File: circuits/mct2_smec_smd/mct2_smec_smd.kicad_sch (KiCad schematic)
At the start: 9 parts, among them J1 Input 1x40 FPC, J2 Conn_01x07, J3 Conn_02x15_Odd_Even, U1 GW1N-UV2QN48C7/I6

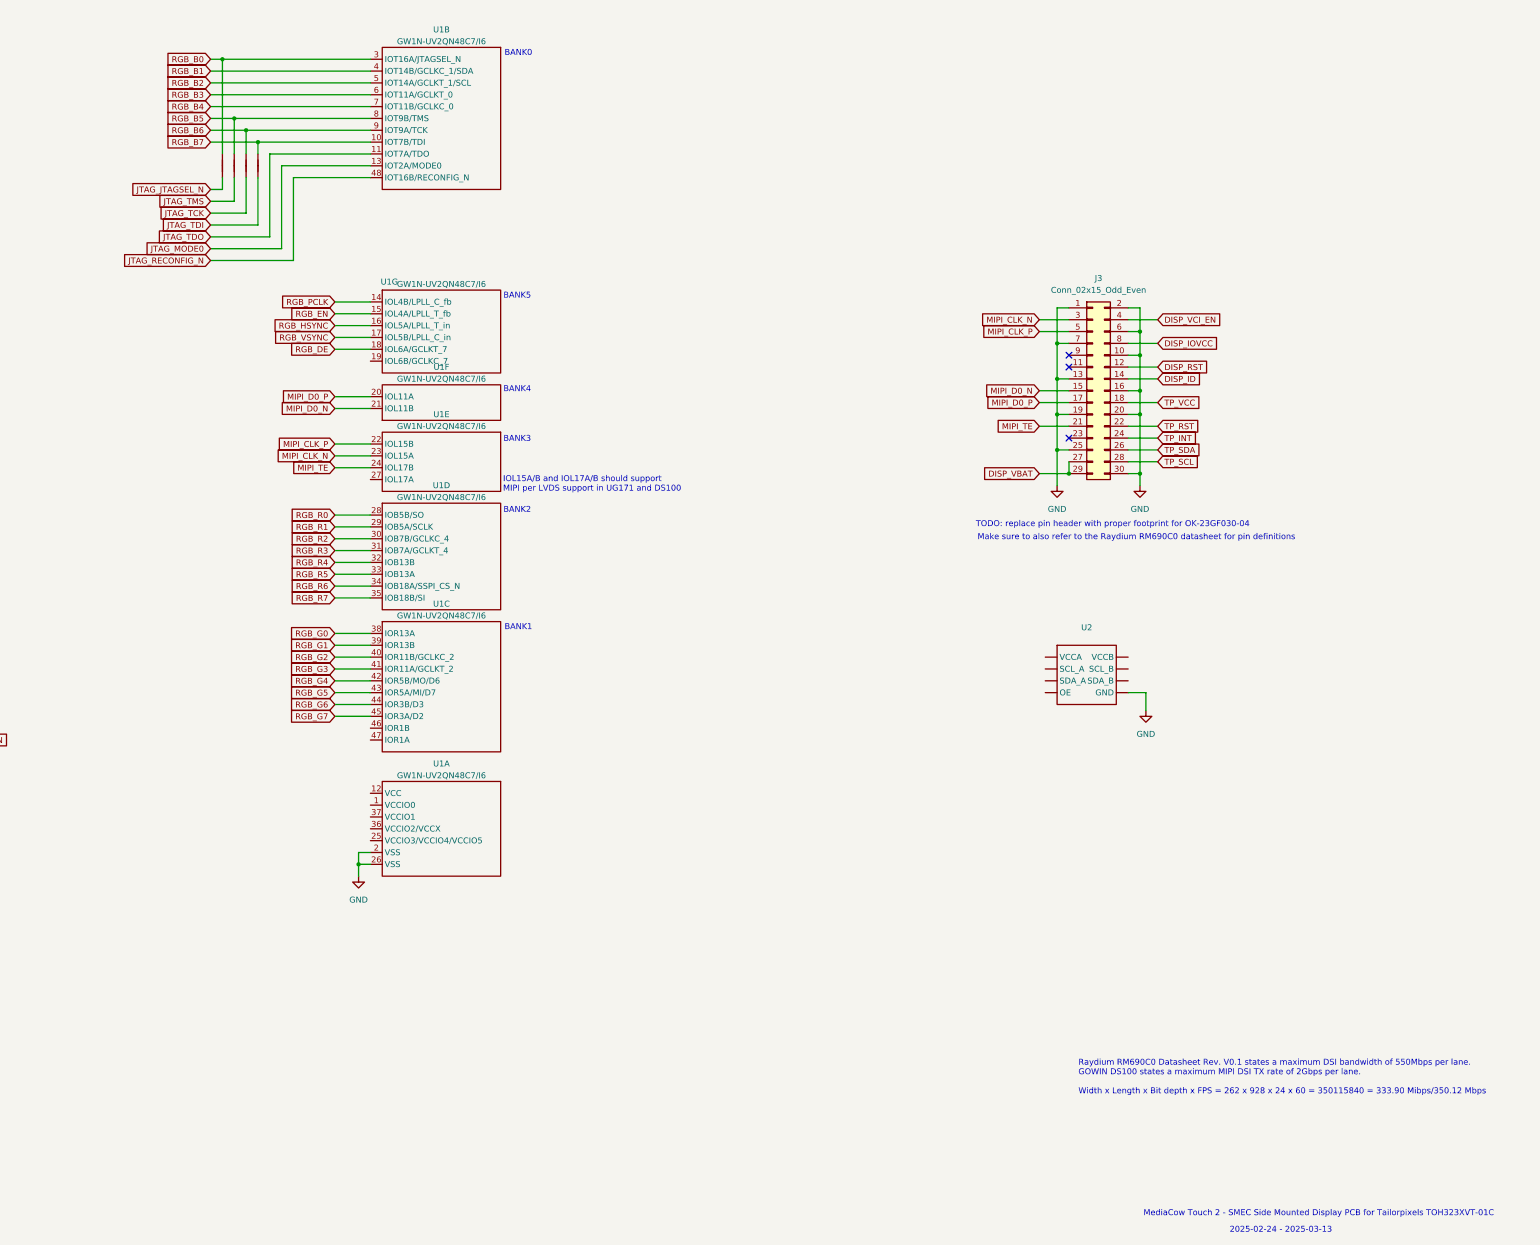
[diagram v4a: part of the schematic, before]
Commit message: 20250316-1
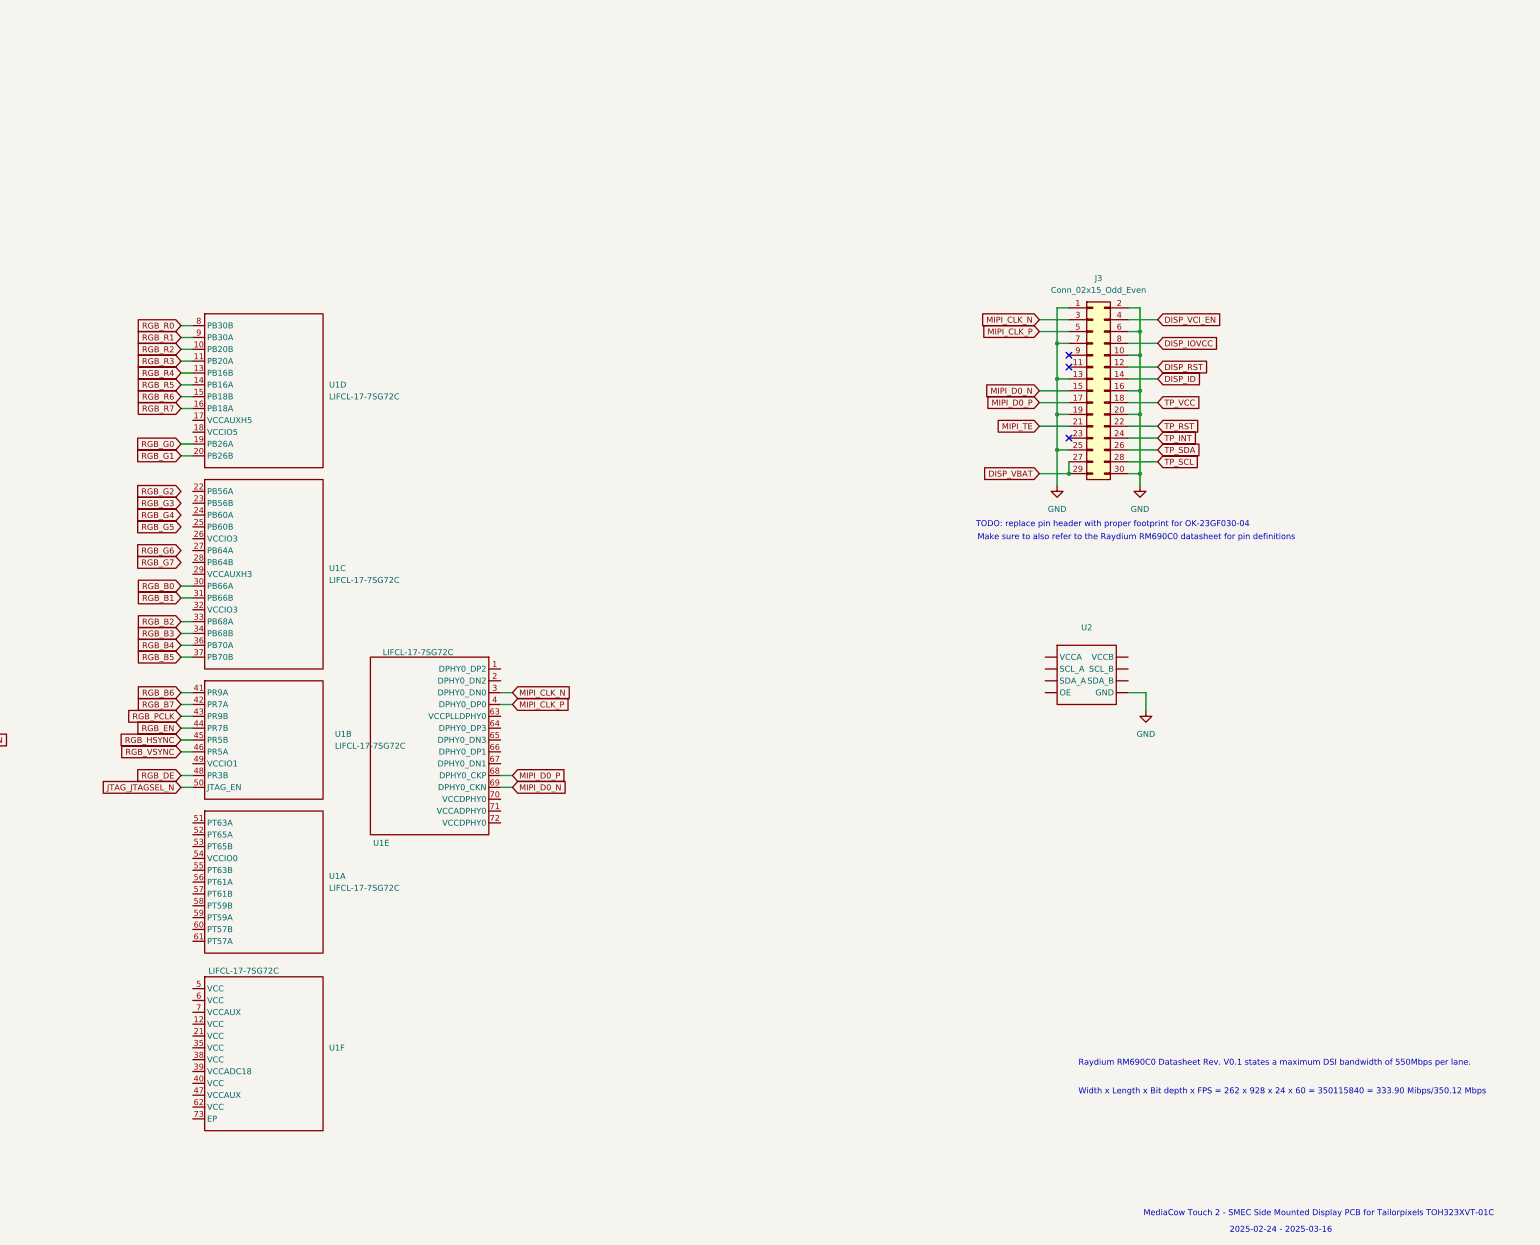
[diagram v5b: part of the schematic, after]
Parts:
- removed NT1, NT2, NT3, NT4: NetTie_2, symbol Device:NetTie_2
- removed U1: GW1N-UV2QN48C7/I6, Package_DFN_QFN:QFN-48-1EP_6x6mm_P0.4mm_EP4.2x4.2mm_ThermalVias, symbol mediacow:GW1N-UV2QN48C7
- added U1: LIFCL-17-7SG72C, Package_DFN_QFN:QFN-72-1EP_10x10mm_P0.5mm_EP6x6mm_ThermalVias, symbol mediacow:LIFCL-17-7SG72C
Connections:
- net JTAG_JTAGSEL_N: now also U1.50 (JTAG_EN)
- net MIPI_CLK_N: now also U1.3 (DPHY0_DN0)
- net MIPI_CLK_P: now also U1.4 (DPHY0_DP0)
- net MIPI_D0_N: now also U1.69 (DPHY0_CKN)
- net MIPI_D0_P: now also U1.68 (DPHY0_CKP)
- net RGB_B0: now also U1.30 (PB66A)
- net RGB_B1: now also U1.31 (PB66B)
- net RGB_B2: now also U1.33 (PB68A)
- net RGB_B3: now also U1.34 (PB68B)
- net RGB_B4: now also U1.36 (PB70A)
- net RGB_B5: now also U1.37 (PB70B)
- net RGB_B6: now also U1.41 (PR9A)
- net RGB_B7: now also U1.42 (PR7A)
- net RGB_DE: now also U1.48 (PR3B)
- net RGB_EN: now also U1.44 (PR7B)
- net RGB_G0: now also U1.19 (PB26A)
- net RGB_G1: now also U1.20 (PB26B)
- net RGB_HSYNC: now also U1.45 (PR5B)
- net RGB_PCLK: now also U1.43 (PR9B)
- net RGB_R0: now also U1.8 (PB30B)
- net RGB_R1: now also U1.9 (PB30A)
- net RGB_R2: now also U1.10 (PB20B)
- net RGB_R3: now also U1.11 (PB20A)
- net RGB_R4: now also U1.13 (PB16B)
- net RGB_R5: now also U1.14 (PB16A)
- net RGB_R6: now also U1.15 (PB18B)
- net RGB_R7: now also U1.16 (PB18A)
- net RGB_VSYNC: now also U1.46 (PR5A)
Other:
- note added: "2025-02-24 - 2025-03-16"
- note added: "Raydium RM690C0 Datasheet Rev. V0.1 states a maximum DSI bandwidth of 550Mbps per lane. Width x Length x Bit depth x FPS = 262 x 928 x 24 x 60 = 350115840 = 333.90 Mibps/350.12 Mbps"
- note removed: "2025-02-24 - 2025-03-13"
- note removed: "BANK0"
- note removed: "BANK1"
- note removed: "BANK2"
- note removed: "BANK3"
- note removed: "BANK4"
- note removed: "BANK5"
- note removed: "IOL15A/B and IOL17A/B should support MIPI per LVDS support in UG171 and DS100"
- note removed: "Raydium RM690C0 Datasheet Rev. V0.1 states a maximum DSI bandwidth of 550Mbps per lane. GOWIN DS100 states a maximum MIPI DSI TX rate of 2Gbps per lane. Width x Length x Bit depth x FPS = 262 x 928 x 24 x 60 = 350115840 = 333.90 Mibps/350.12 Mbps"
